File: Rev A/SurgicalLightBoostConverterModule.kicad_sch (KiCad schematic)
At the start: 44 parts, among them Q1 BC337, Q2 IRLZ44N, Q3 BC327, Q4 IRLZ44N, Q5 BC327, U1 TL494, U2 TL431D, U3 LM358

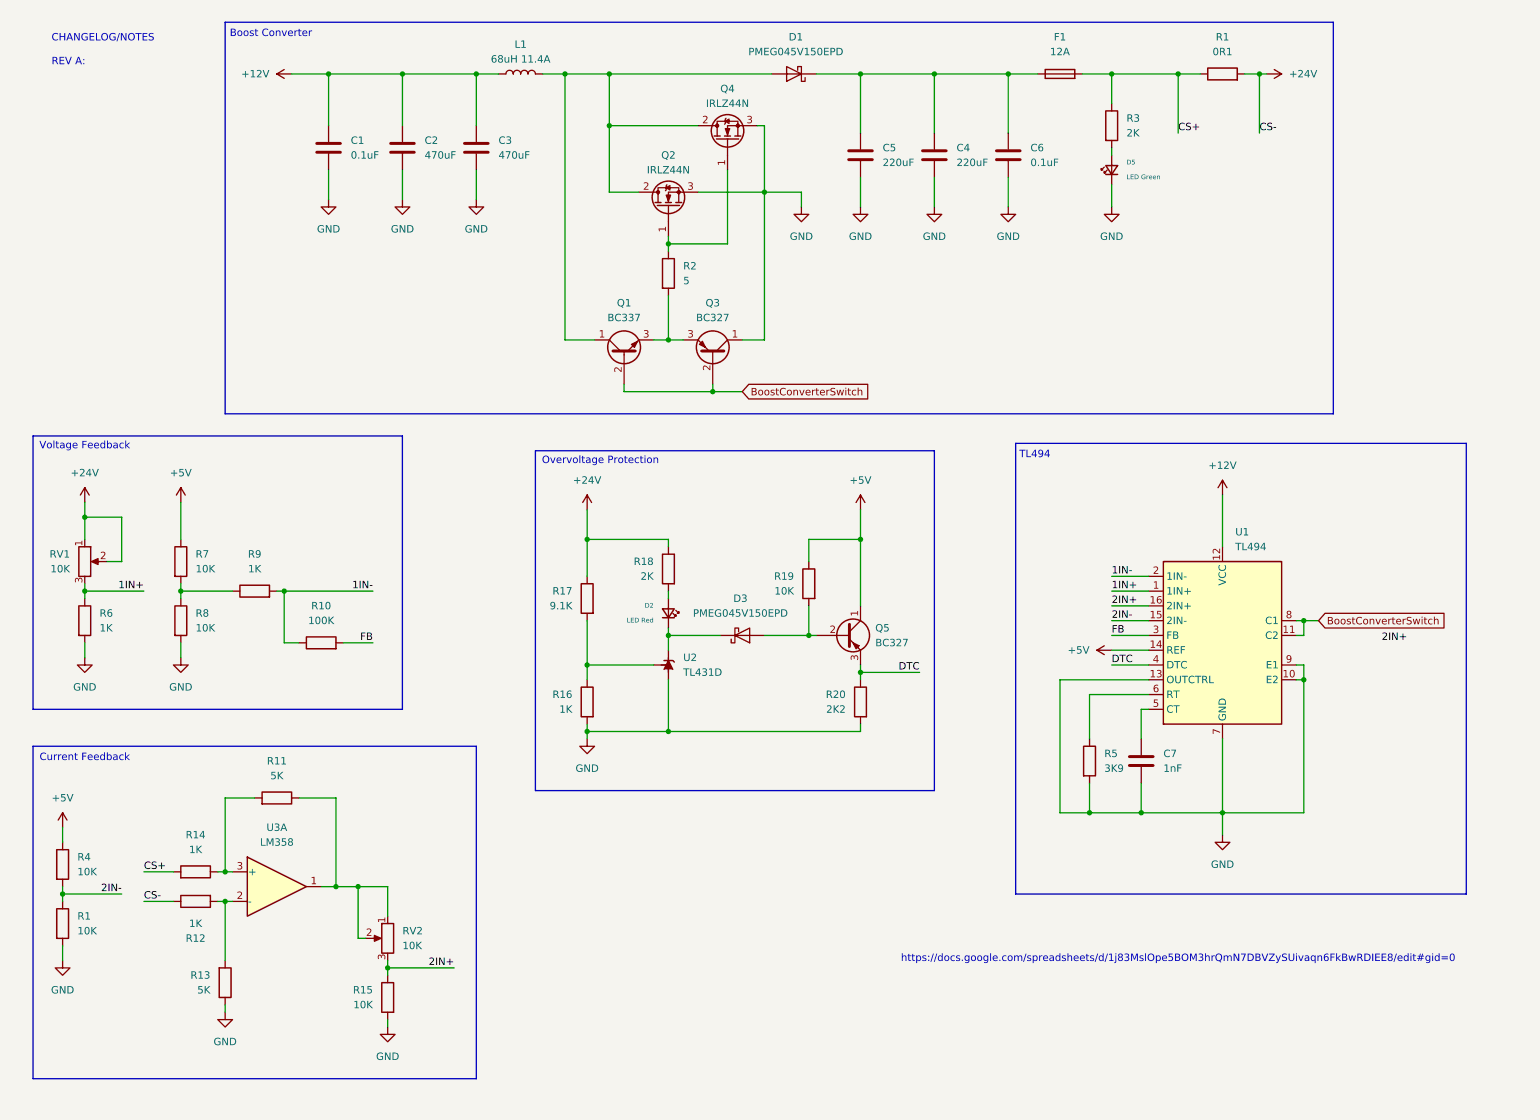
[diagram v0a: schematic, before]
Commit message: More schematic updates.
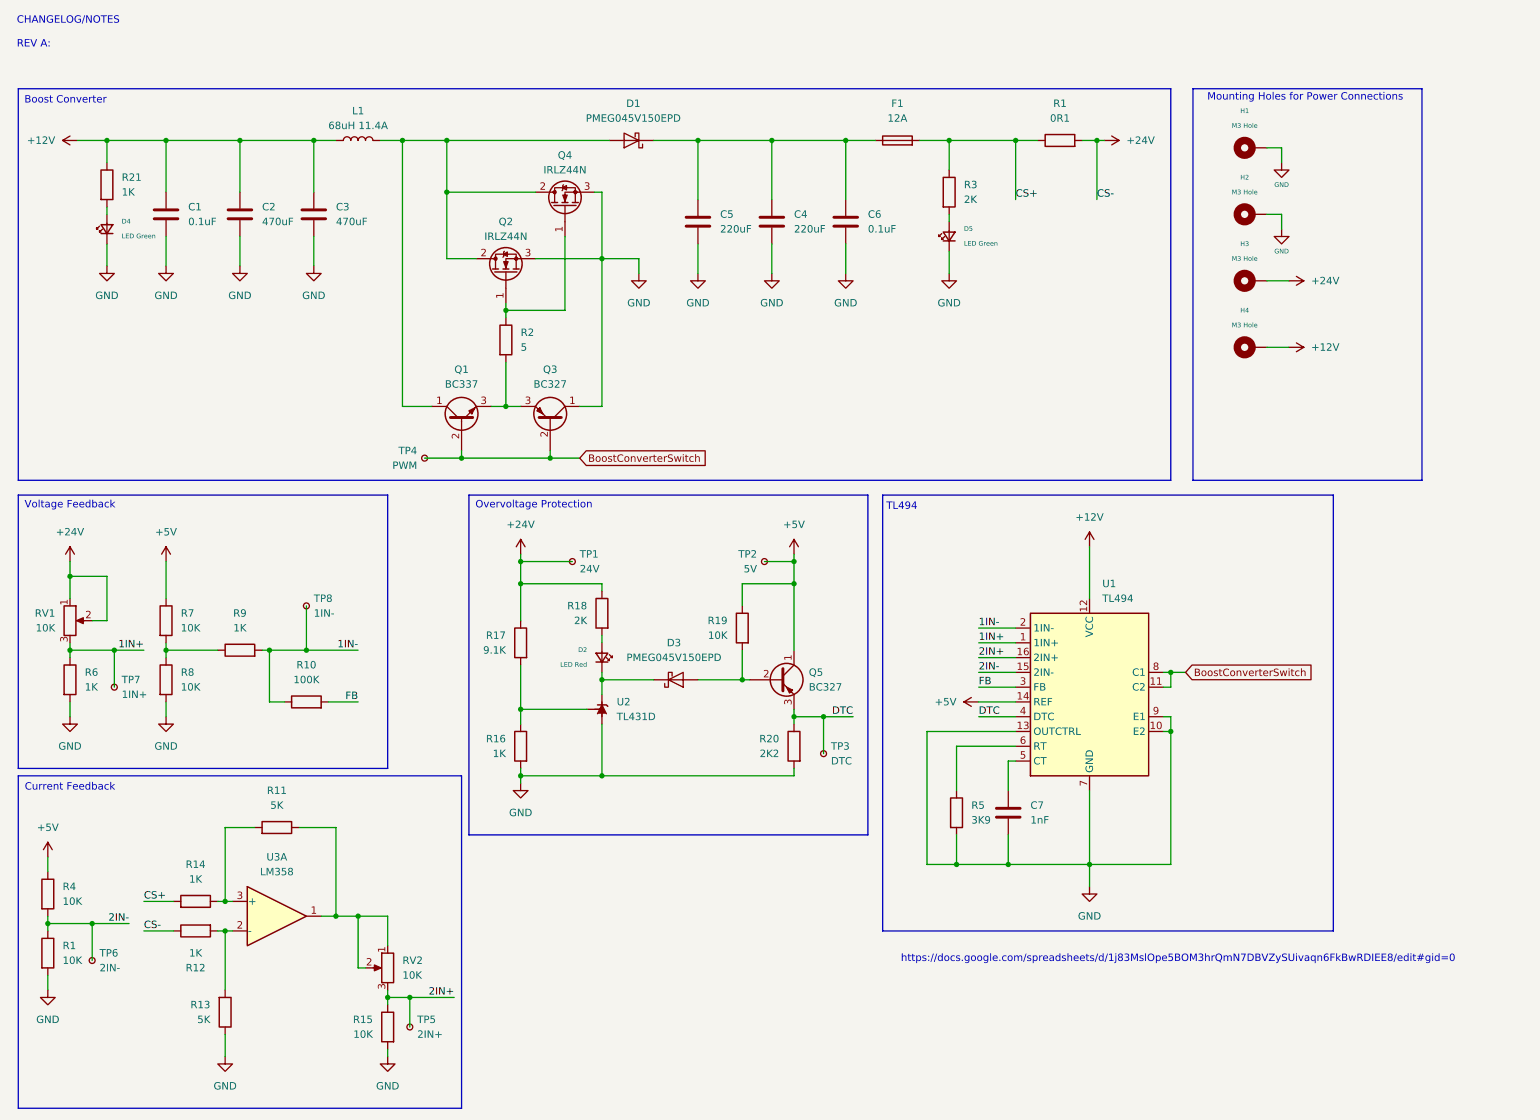
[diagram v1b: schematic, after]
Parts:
- added D4: LED Green, LED_SMD:LED_0805_2012Metric, symbol Device:LED_Small
- added H1, H2, H3, H4: M3 Hole, MountingHole:MountingHole_3.2mm_M3_Pad_TopBottom, symbol Mechanical:MountingHole_Pad
- added R21: 1K, Resistor_SMD:R_0805_2012Metric, symbol Device:R
- added TP1: 24V, symbol Connector:TestPoint_Small
- added TP2: 5V, symbol Connector:TestPoint_Small
- added TP3: DTC, symbol Connector:TestPoint_Small
- added TP4: PWM, symbol Connector:TestPoint_Small
- added TP5: 2IN+, symbol Connector:TestPoint_Small
- added TP6: 2IN-, symbol Connector:TestPoint_Small
- added TP7: 1IN+, symbol Connector:TestPoint_Small
- added TP8: 1IN-, symbol Connector:TestPoint_Small
- C2, C3: footprint (none) -> Capacitor_THT:CP_Radial_D12.5mm_P5.00mm
- C4, C5: footprint (none) -> Capacitor_THT:CP_Radial_D10.0mm_P5.00mm
- L1: footprint (none) -> Inductor_THT:L_Radial_D29.8mm_P29.30mm_Murata_1400series
- RV1, RV2: footprint (none) -> Connector_PinHeader_2.54mm:PinHeader_1x03_P2.54mm_Vertical
- U1: footprint (none) -> Package_DIP:DIP-16_W7.62mm
- U3: footprint (none) -> Package_DIP:DIP-8_W7.62mm_Socket
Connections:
- net +12V: now also H4.1, R21.1
- net +24V: now also H3.1, TP1.1
- net +5V: now also TP2.1
- net 1IN+: now also TP7.1
- net 1IN-: now also TP8.1
- net 2IN+: now also TP5.1
- net 2IN-: now also TP6.1
- net BoostConverterSwitch: now also TP4.1
- net DTC: now also TP3.1
- net GND: now also D4.1 (K), H1.1, H2.1
- new net: D4.2 (A), R21.2
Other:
- note added: "Mounting Holes for Power Connections"
- moved on the sheet: C1, C2, C4, C5, C6, C7, D1, D2, D3, D5, F1, L1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
